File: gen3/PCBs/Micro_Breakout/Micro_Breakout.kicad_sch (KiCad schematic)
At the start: 46 parts, among them J1 430450422, J10 430450228, J11 430450422, J12 430450228, J13 430450228, J14 Conn_01x03_Pin, J15 430450422, J16 430450422, J17 430450422, J18 430450422, J19 Conn_01x10, J2 SBH11-PBPC-D05-ST-BK, J20 Conn_01x10, J21 Conn_01x10, J22 430450612, J23 430450612, J24 430450612, J25 430450422, J3 Battery, J4 Conn_01x24, J5 Battery, J6 Conn_01x24, J7 430450422, J8 430450422, J9 430450228, Q7 L78M05ABDT-TR, U15 AMS1117-3.3, U2 MCP9808_MSOP, U4 BME280, U6 Teensy4.1

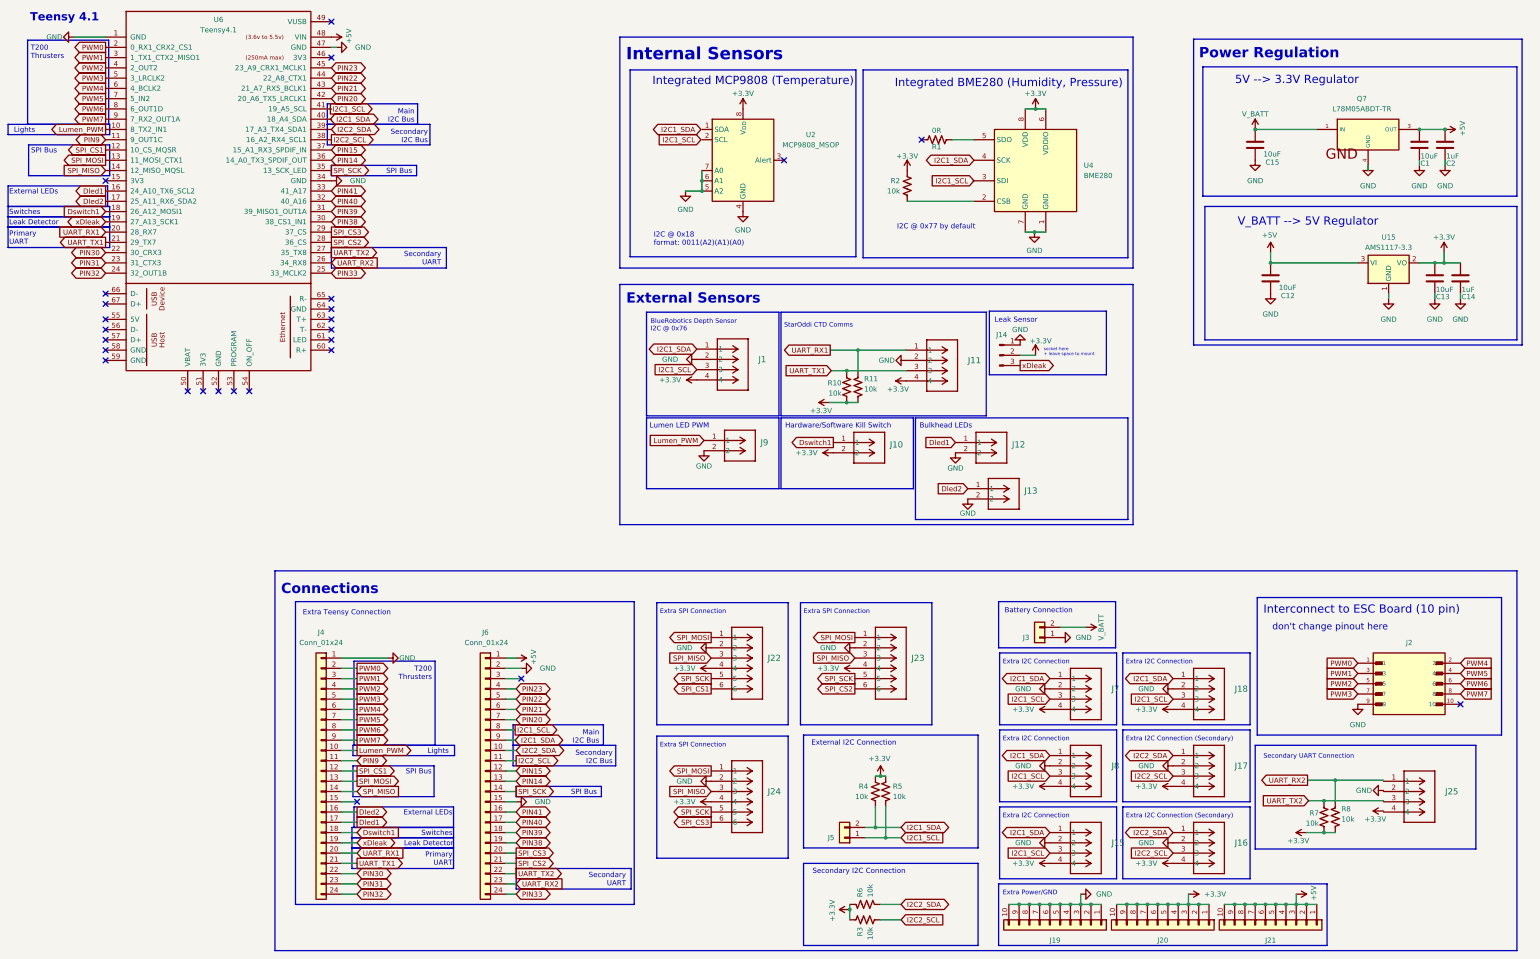
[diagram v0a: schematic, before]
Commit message: microcontroller breakout board completed!!
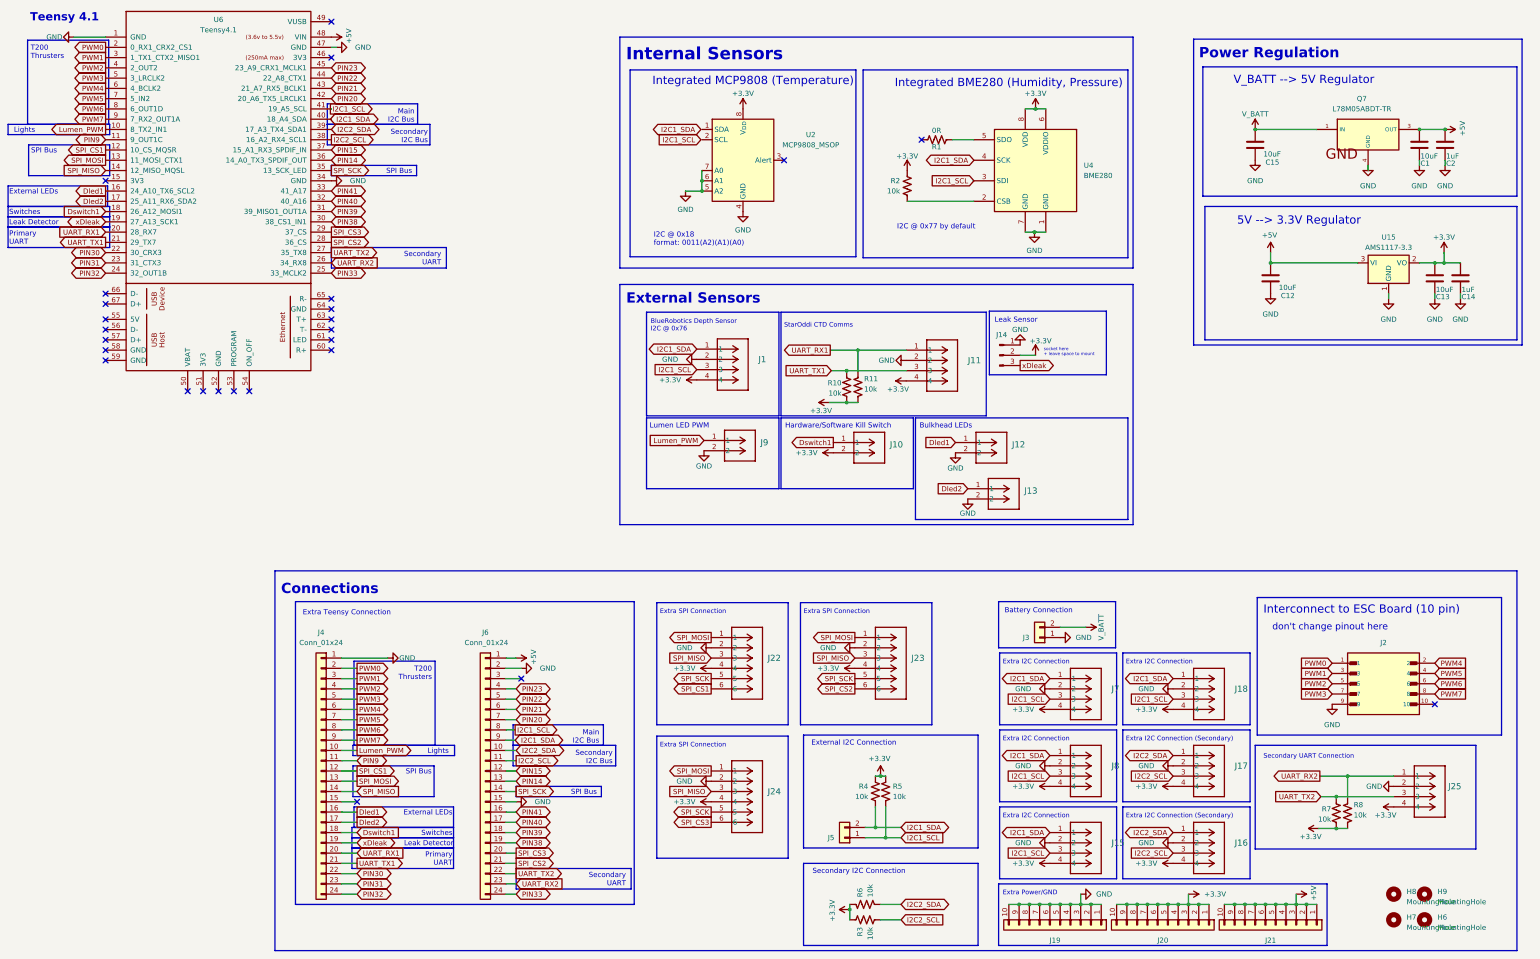
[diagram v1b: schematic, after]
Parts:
- added H6, H7, H8, H9: MountingHole, MountingHole:MountingHole_4.3mm_M4, symbol Mechanical:MountingHole
- J1: value 430450422 -> BlueRobotics Depth Sensor
- J10: value 430450228 -> Kill Switch
- J11: value 430450422 -> StarOddi CTD Comms
- J12: value 430450228 -> LED1
- J13: value 430450228 -> LED2
- J14: value Conn_01x03_Pin -> Leak Sensor
- J15: value 430450422 -> Extra I2C #3
- J16: value 430450422 -> Extra I2C #6
- J17: value 430450422 -> Extra I2C #5
- J18: value 430450422 -> Extra I2C #4
- J19: value Conn_01x10 -> GND Line
- J2: value SBH11-PBPC-D05-ST-BK -> Interconnect
- J20: value Conn_01x10 -> 3.3V Line
- J21: value Conn_01x10 -> 5V Line
- J22: value 430450612 -> Extra SPI #1
- J23: value 430450612 -> Extra SPI #2
- J24: value 430450612 -> Extra SPI #3
- J25: value 430450422 -> Secondary UART
- J3: value Battery -> External Battery
- J5: value Battery -> External I2C
- J7: value 430450422 -> Extra I2C #1
- J8: value 430450422 -> Extra I2C #2
- J9: value 430450228 -> Lumen PWM
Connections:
- net +3.3V: now also J25.4
- net Dled1: now also J4.16 (Pin_16); no longer J4.17 (Pin_17)
- net Dled2: now also J4.17 (Pin_17); no longer J4.16 (Pin_16)
- net GND: now also J25.2
- net UART_RX2: now also J25.1
- net UART_TX2: now also J25.3
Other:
- moved on the sheet: J2, J25, R7, R8
